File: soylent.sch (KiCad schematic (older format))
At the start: 17 parts, among them J1 DB9_Female, J2 Conn_01x04, J3 Conn_01x04, J4 Conn_02x03_Counter_Clockwise, Q1 BC847BPN, U1 ATtiny202-SS, U2 MIC5504-3.3YM5

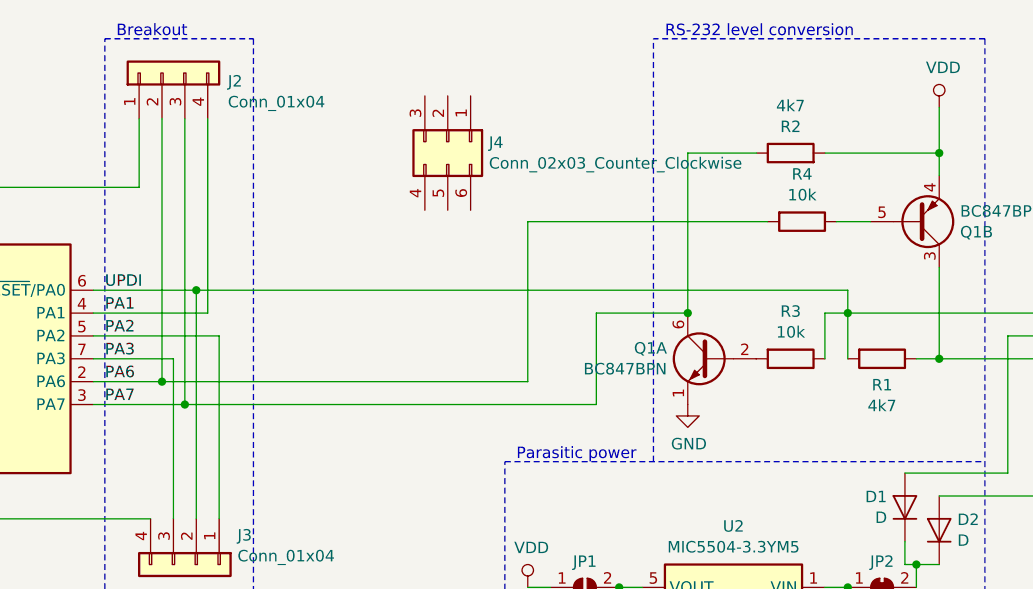
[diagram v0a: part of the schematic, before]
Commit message: Cleanup and prep for TTY I/F
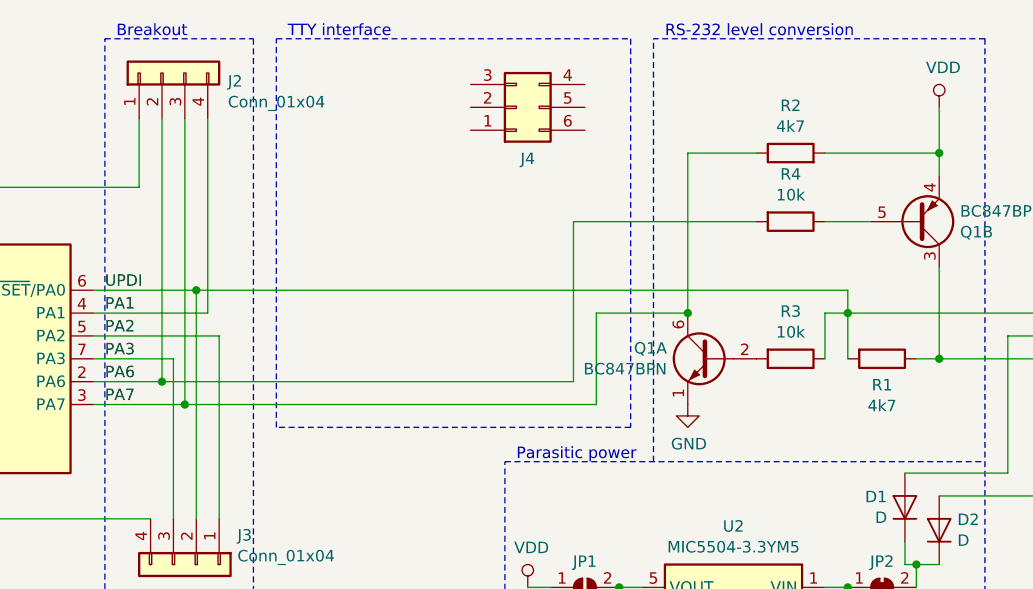
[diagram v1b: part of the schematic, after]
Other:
- note added: "TTY interface"
- moved on the sheet: J4, R4
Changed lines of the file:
@@
 L Connector_Generic:Conn_02x03_Counter_Clockwise J4
 U 1 1 5DDE85A2
-P 5900 2850
-F 0 "J4" V 5904 3030 50  0000 L CNN
-F 1 "Conn_02x03_Counter_Clockwise" V 5995 3030 50  0000 L CNN
-F 2 "Pin_Headers:Pin_Header_Straight_2x03_Pitch2.54mm" H 5900 2850 50  0001 C CNN
-F 3 "~" H 5900 2850 50  0001 C CNN
-	1    5900 2850
-	0    1    1    0
+P 6200 2700
+F 0 "J4" H 6250 2925 50  0000 C CNN
+F 1 "Conn_02x03_Counter_Clockwise" V 6295 2880 50  0001 L CNN
+F 2 "Pin_Headers:Pin_Header_Straight_2x03_Pitch2.54mm" H 6200 2700 50  0001 C CNN
+F 3 "~" H 6200 2700 50  0001 C CNN
+	1    6200 2700
+	1    0    0    1
 $EndComp
 Wire Wire Line
@@
 U 1 1 5DDFC6FD
 P 7400 2900
-F 0 "R2" V 7515 2900 50  0000 C CNN
-F 1 "4k7" V 7606 2900 50  0000 C CNN
+F 0 "R2" V 7607 2900 50  0000 C CNN
+F 1 "4k7" V 7516 2900 50  0000 C CNN
 F 2 "Resistors_SMD:R_0603_HandSoldering" V 7330 2900 50  0001 C CNN
 F 3 "~" H 7400 2900 50  0001 C CNN
@@
 	1    0    0    -1
 $EndComp
-Wire Wire Line
-	4650 3900 6250 3900
 Connection ~ 4650 3900
 Wire Wire Line
@@
 	8050 3400 8050 3800
 Connection ~ 6950 3600
-Wire Wire Line
-	6250 3900 6250 3200
 Wire Wire Line
 	6950 2900 7250 2900
@@
 L Device:R R4
 U 1 1 5DDEECC2
-P 7450 3200
-F 0 "R4" V 7243 3200 50  0000 C CNN
-F 1 "10k" V 7334 3200 50  0000 C CNN
-F 2 "Resistors_SMD:R_0603_HandSoldering" V 7380 3200 50  0001 C CNN
-F 3 "~" H 7450 3200 50  0001 C CNN
-	1    7450 3200
+P 7400 3200
+F 0 "R4" V 7193 3200 50  0000 C CNN
+F 1 "10k" V 7284 3200 50  0000 C CNN
+F 2 "Resistors_SMD:R_0603_HandSoldering" V 7330 3200 50  0001 C CNN
+F 3 "~" H 7400 3200 50  0001 C CNN
+	1    7400 3200
 	0    1    1    0
 $EndComp
-Wire Wire Line
-	7750 3200 7600 3200
-Wire Wire Line
-	6250 3200 7300 3200
 $Comp
 L Device:R R3
@@
 Text Notes 6200 4250 0    50   ~ 0
 Parasitic power
+Wire Notes Line
+	5150 2400 6700 2400
+Wire Notes Line
+	6700 2400 6700 4100
+Wire Notes Line
+	6700 4100 5150 4100
+Wire Notes Line
+	5150 4100 5150 2400
+Wire Wire Line
+	6450 3900 6450 3200
+Wire Wire Line
+	6450 3200 7250 3200
+Wire Wire Line
+	4650 3900 6450 3900
+Wire Wire Line
+	7550 3200 7750 3200
+Text Notes 5200 2400 0    50   ~ 0
+TTY interface
 $EndSCHEMATC
